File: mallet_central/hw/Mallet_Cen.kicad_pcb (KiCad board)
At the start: 2 copper layers, 41 x 19.8 mm, 25 parts, among them J1 Barrel_Jack_Switch_Pin3Ring, J2 Conn_01x04, J3 Conn_01x08, J4 Conn_01x04, U1 MT2492, U2 STM32G030F6Px, U3 LTC4311CSC6#TRPBF

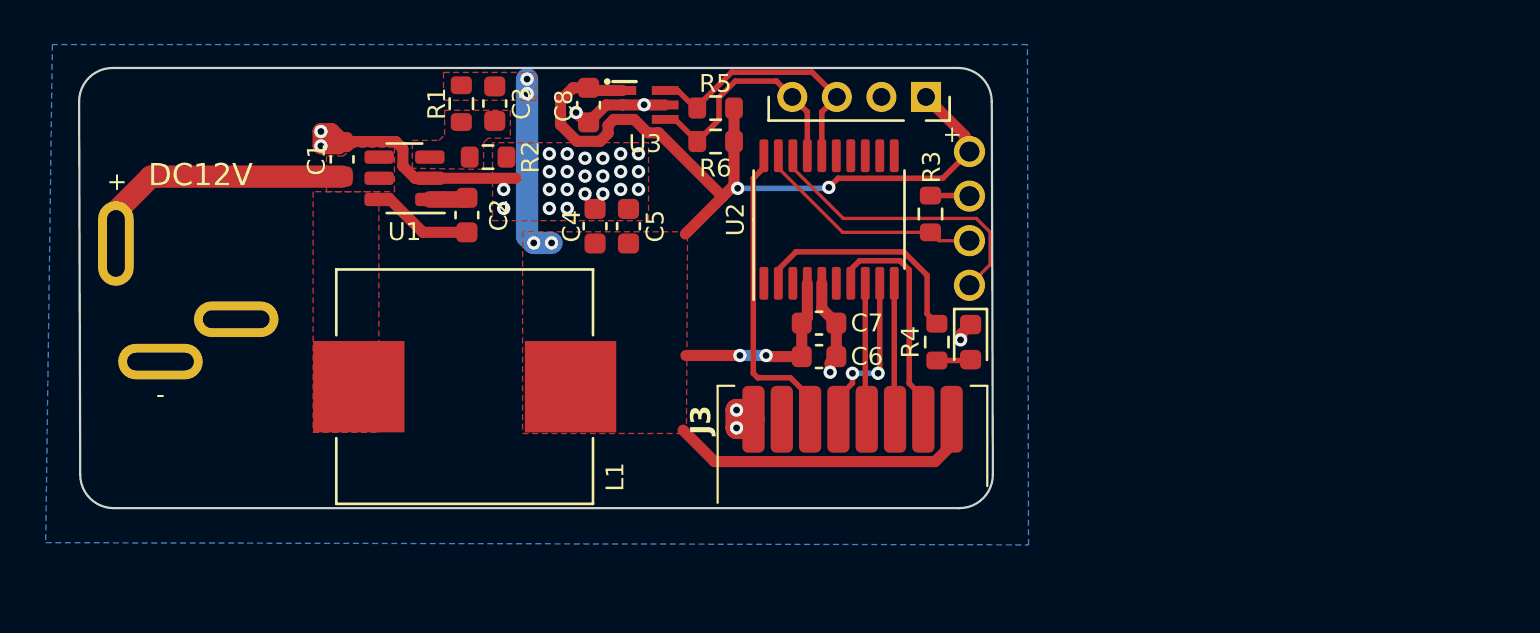
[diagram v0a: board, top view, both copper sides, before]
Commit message: Revise central module hardware design
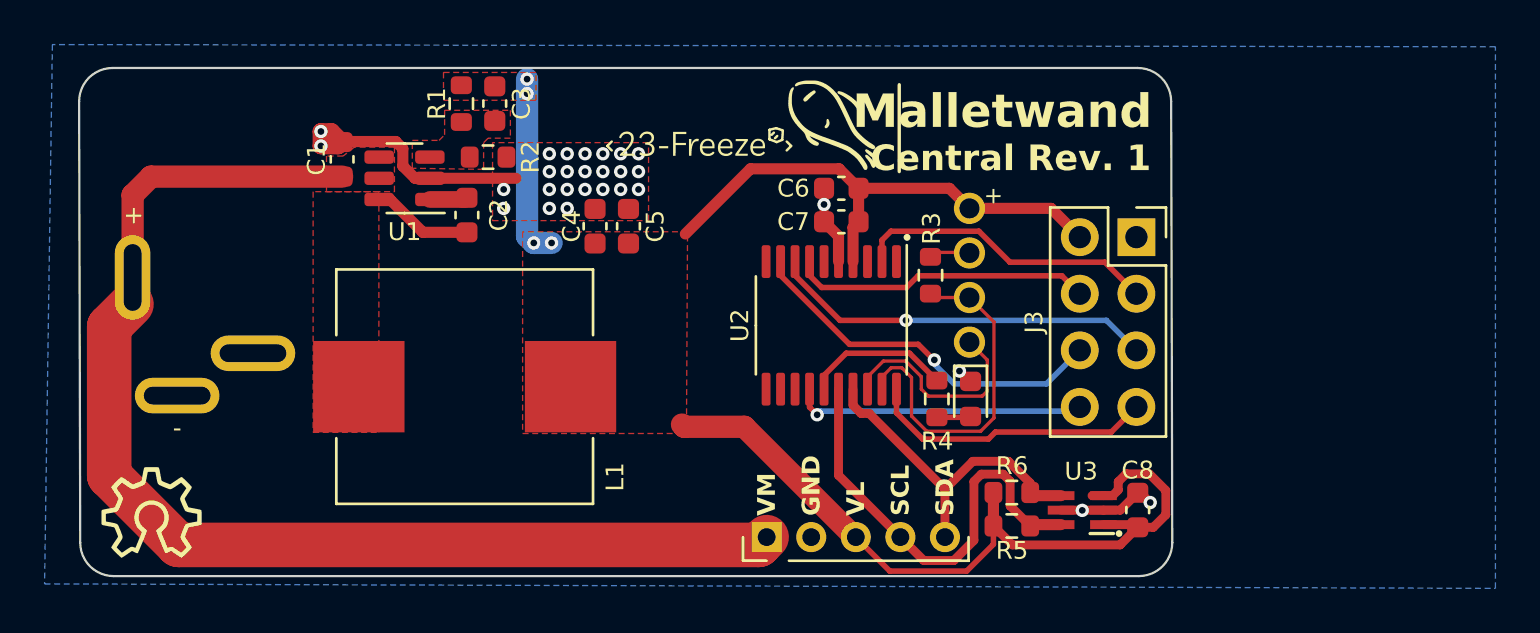
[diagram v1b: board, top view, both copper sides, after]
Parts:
- added G***: LOGO, LOGO, F.Cu at (40.3, 75.4)
- G*** (x2): moved to F.Cu
- J3: value Conn_01x08 -> Conn_02x04_Odd_Even; footprint Mallet_Cen_footprints:SMD_Module_P1.27_1x08 -> Connector_PinSocket_2.54mm:PinSocket_2x04_P2.54mm_Vertical
- J4: value Conn_01x04 -> Conn_01x05; footprint Connector_PinHeader_2.00mm:PinHeader_1x04_P2.00mm_Vertical -> Connector_PinHeader_2.00mm:PinHeader_1x05_P2.00mm_Vertical
- moved G*** 31.5 mm to (71.0, 58.1), turned to 0 degrees
- moved C8 30.6 mm to (84.5, 75.3), turned to 90 degrees
- moved U3 26.8 mm to (82.1, 75.3), turned to 180 degrees
- moved R5 23.0 mm to (78.9, 76.0), turned to 0 degrees
- moved J4 21.0 mm to (67.9, 76.5), turned to 90 degrees
- moved R6 20.6 mm to (78.9, 74.5), turned to 0 degrees
- moved G*** 19.3 mm to (64.5, 58.9), turned to 0 degrees
- moved J3 11.6 mm to (84.5, 63.1), turned to 0 degrees
- moved C6 7.62 mm to (71.2, 60.9), turned to 180 degrees
- moved U2 4.75 mm to (70.8, 67.0), turned to -90 degrees
- moved C7 4.66 mm to (71.2, 62.4), turned to 180 degrees
- moved R3 2.75 mm to (75.2, 64.8)
- moved D2 2.55 mm to (77.0, 70.3)
- moved J2 2.55 mm to (77.0, 64.8)
- moved R4 2.55 mm to (75.5, 70.3)
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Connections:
- J3 pad 1: VDD -> GND
- J3 pad 2: nRF_CE -> VDD
- J3 pad 3: SPI1_CSx -> nRF_CE
- J3 pad 4: SPI1_CK -> nRF_CS
- J3 pad 5: SPI1_MOSI -> SPI1_SCK
- J3 pad 6: SPI1_MISO -> SPI1_MOSI
- J3 pad 7: unconnected-(J3-Pin_7-Pad7) -> SPI1_MISO
- J3 pad 8: GND -> nRF_IRQ
- J4 pad 1: VDD -> VBUS
- J4 pad 3: I2C2_SCL -> VDD
- J4 pad 4: I2C2_SDA -> I2C2_SCL
- U2 pad 10: SPI1_CSx -> unconnected-(U2-PA3-Pad10)
- U2 pad 14: unconnected-(U2-PA7-Pad14) -> nRF_IRQ
- U2 pad 15: unconnected-(U2-PB0/PB1/PB2/PA8-Pad15) -> ACT_LED
- U2 pad 2: ACT_LED -> nRF_CE
- U2 pad 7: nRF_CE -> nRF_CS
- U2 pad 8: SPI1_CK -> SPI1_SCK
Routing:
- net VBUS: track 12.2 -> 51.0 mm
- net SPI1_SCK: track 0.00 -> 17.3 mm, vias 0 -> 1
- net nRF_CS: track 0.00 -> 13.5 mm
- net nRF_IRQ: track 0.00 -> 13.2 mm, vias 0 -> 1
- net SPI1_MOSI: track 7.54 -> 16.8 mm, vias 2 -> 1
- net I2C2_SCL: track 12.1 -> 20.2 mm
- net SPI1_CK: track 6.13 -> 0.00 mm
- net SPI1_CSx: track 6.11 -> 0.00 mm
- net SWCLK: track 10.5 -> 16.0 mm
- net I2C2_SDA: track 11.0 -> 15.2 mm
- net ACT_LED: track 10.4 -> 6.60 mm
- net GND: track 26.0 -> 22.3 mm, vias 30 -> 28
- net SWDIO: track 13.4 -> 9.82 mm
- net nRF_CE: track 10.5 -> 13.7 mm
- net VDD: track 65.9 -> 66.9 mm, vias 8 -> 4
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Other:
- board size 41 x 19.8 mm -> 49 x 22.8 mm
- board text added: "Central Rev. 1"
- board text added: "Malletwand"
- board text added: "VL"
- board text added: "VM"
- board text removed: "DC12V"
